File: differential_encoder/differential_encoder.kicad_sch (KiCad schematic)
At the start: 43 parts, among them J101 Conn_01x12, J102 RJ45_LED_Shielded, J103 RJ45_LED_Shielded, Q101 Q_NMOS_GSD, Q102 Q_NMOS_GSD, Q103 Q_NMOS_GSD, Q104 Q_NMOS_GSD, Q105 Q_NMOS_GSD, Q106 Q_NMOS_GSD, U101 MAX489E, U102 MAX489E, U103 MAX489E, U104 MAX489E, U105 MAX489E, U106 MAX489E

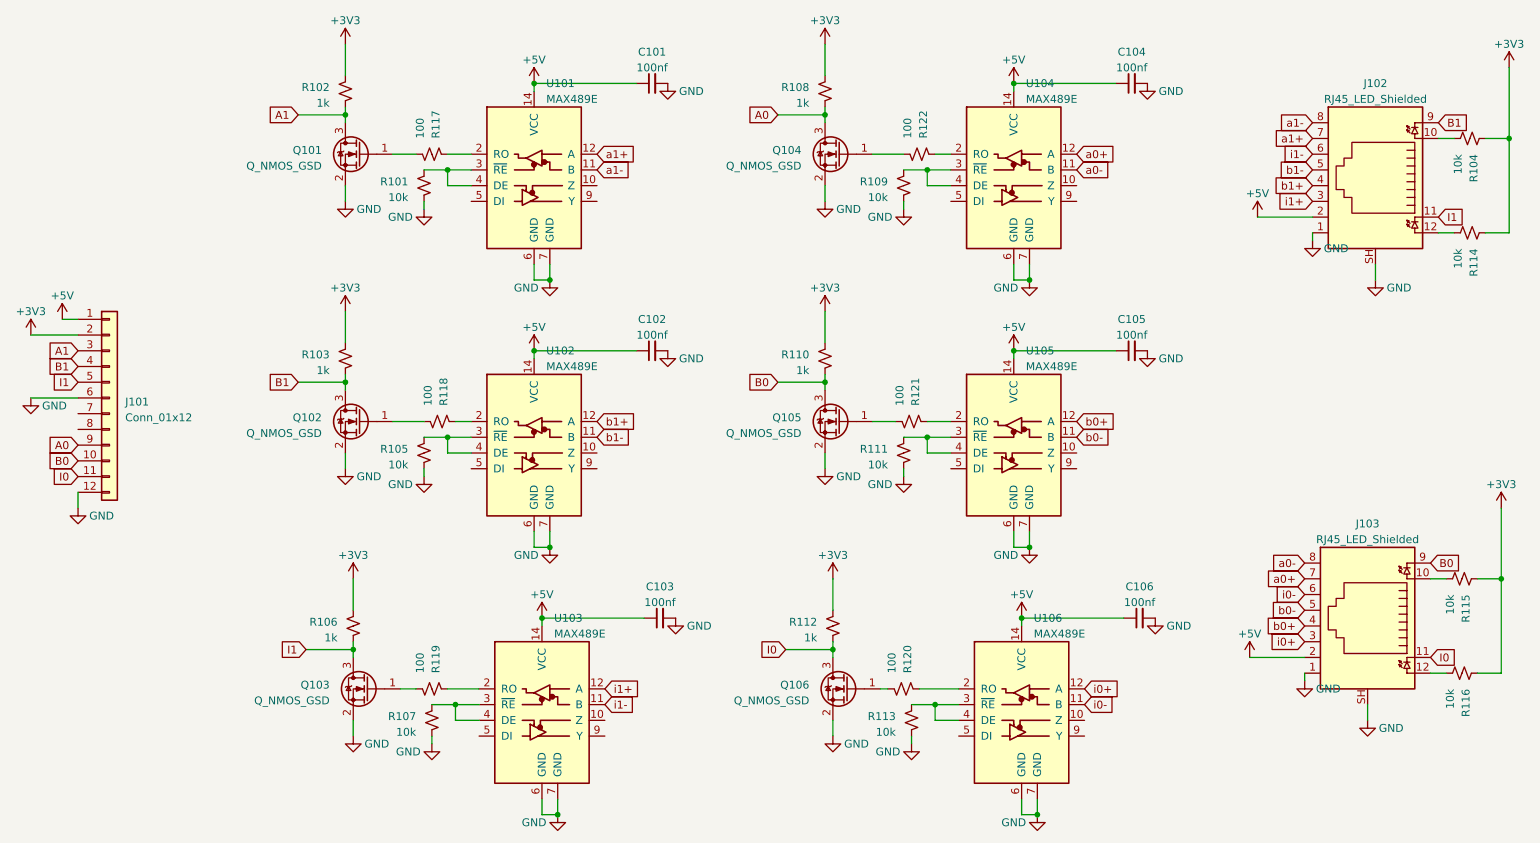
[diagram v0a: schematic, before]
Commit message: final version odrive
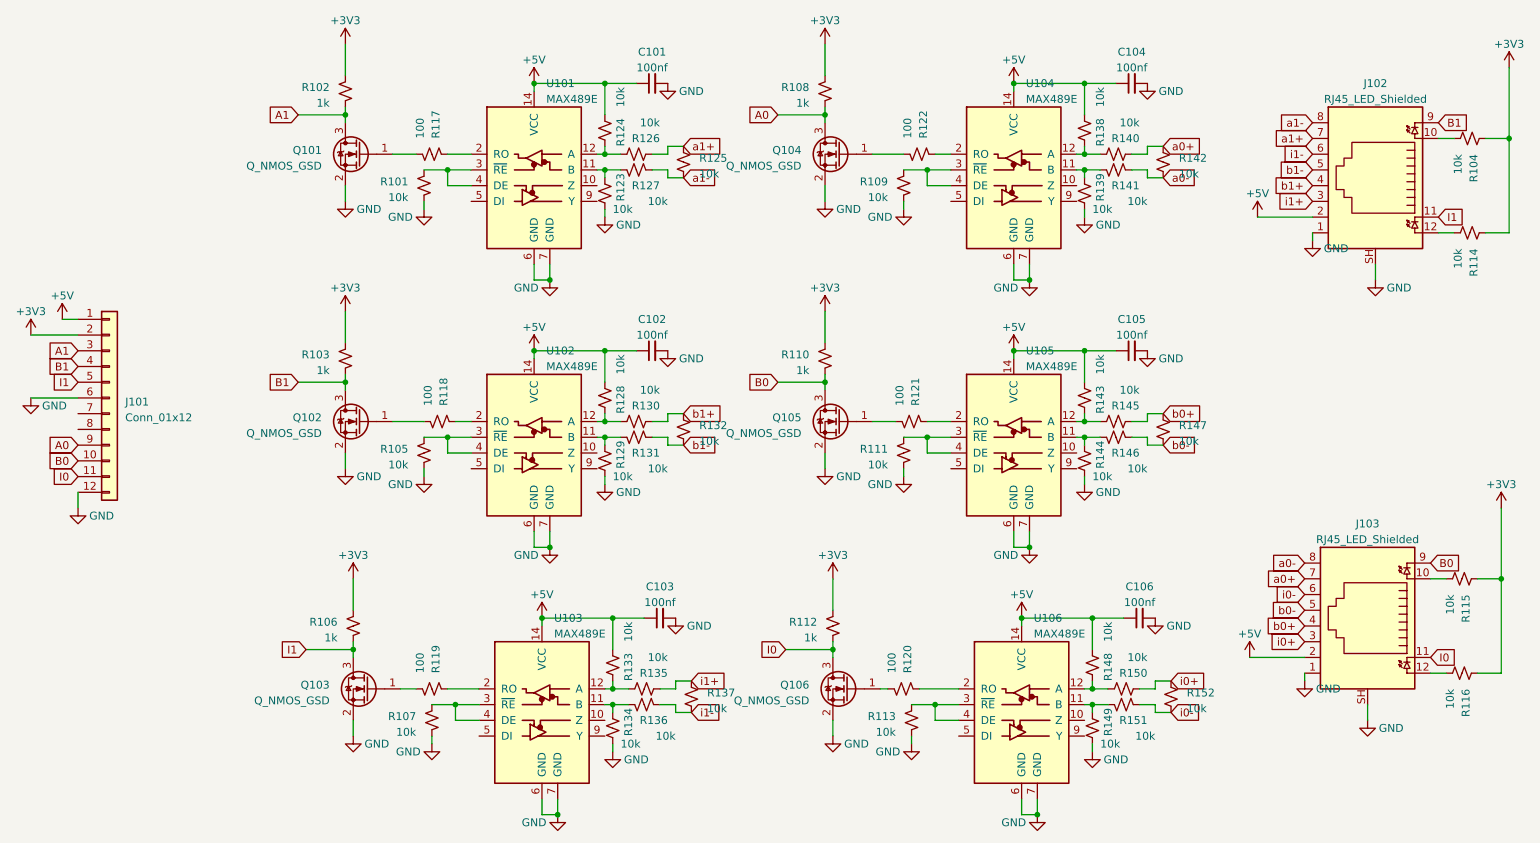
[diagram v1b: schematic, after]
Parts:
- added R123, R124, R125, R126, R127, R128, R129, R130, R131, R132, R133, R134, R135, R136, R137, R138, R139, R140, R141, R142, R143, R144, R145, R146, R147, R148, R149, R150, R151, R152: 10k, Resistor_SMD:R_0805_2012Metric_Pad1.20x1.40mm_HandSolder, symbol Device:R_Small_US
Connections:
- net +5V: now also R124.1, R128.1, R133.1, R138.1, R143.1, R148.1
- net GND: now also R123.2, R129.2, R134.2, R139.2, R144.2, R149.2
- net a0+: now also R140.2, R142.1; no longer U104.12 (A)
- net a0-: now also R141.2, R142.2; no longer U104.11 (B)
- net a1+: now also R125.1, R126.2; no longer U101.12 (A)
- net a1-: now also R125.2, R127.2; no longer U101.11 (B)
- net b0+: now also R145.2, R147.1; no longer U105.12 (A)
- net b0-: now also R146.2, R147.2; no longer U105.11 (B)
- net b1+: now also R130.2, R132.1; no longer U102.12 (A)
- net b1-: now also R131.2, R132.2; no longer U102.11 (B)
- net i0+: now also R150.2, R152.1; no longer U106.12 (A)
- net i0-: now also R151.2, R152.2; no longer U106.11 (B)
- net i1+: now also R135.2, R137.1; no longer U103.12 (A)
- net i1-: now also R136.2, R137.2; no longer U103.11 (B)
- new net: R134.1, R136.1, U103.11 (B)
- new net: R133.2, R135.1, U103.12 (A)
- new net: R143.2, R145.1, U105.12 (A)
- new net: R148.2, R150.1, U106.12 (A)
- new net: R144.1, R146.1, U105.11 (B)
- new net: R128.2, R130.1, U102.12 (A)
- new net: R138.2, R140.1, U104.12 (A)
- new net: R123.1, R127.1, U101.11 (B)
- new net: R139.1, R141.1, U104.11 (B)
- new net: R124.2, R126.1, U101.12 (A)
- new net: R149.1, R151.1, U106.11 (B)
- new net: R129.1, R131.1, U102.11 (B)
